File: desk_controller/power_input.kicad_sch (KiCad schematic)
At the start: 14 parts, among them J5 Barrel_Jack_MountingPin, U1 BD95831MUV

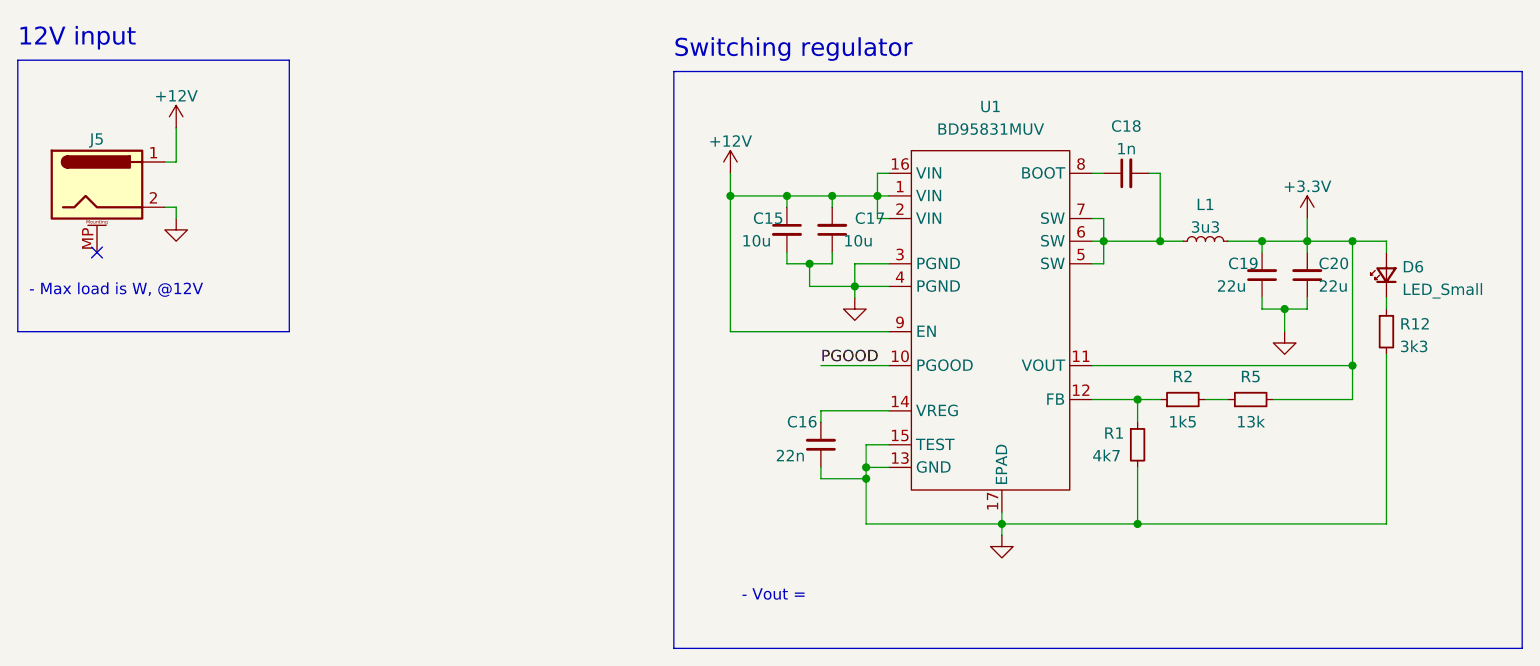
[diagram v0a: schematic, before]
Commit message: Much progress in sch and brd
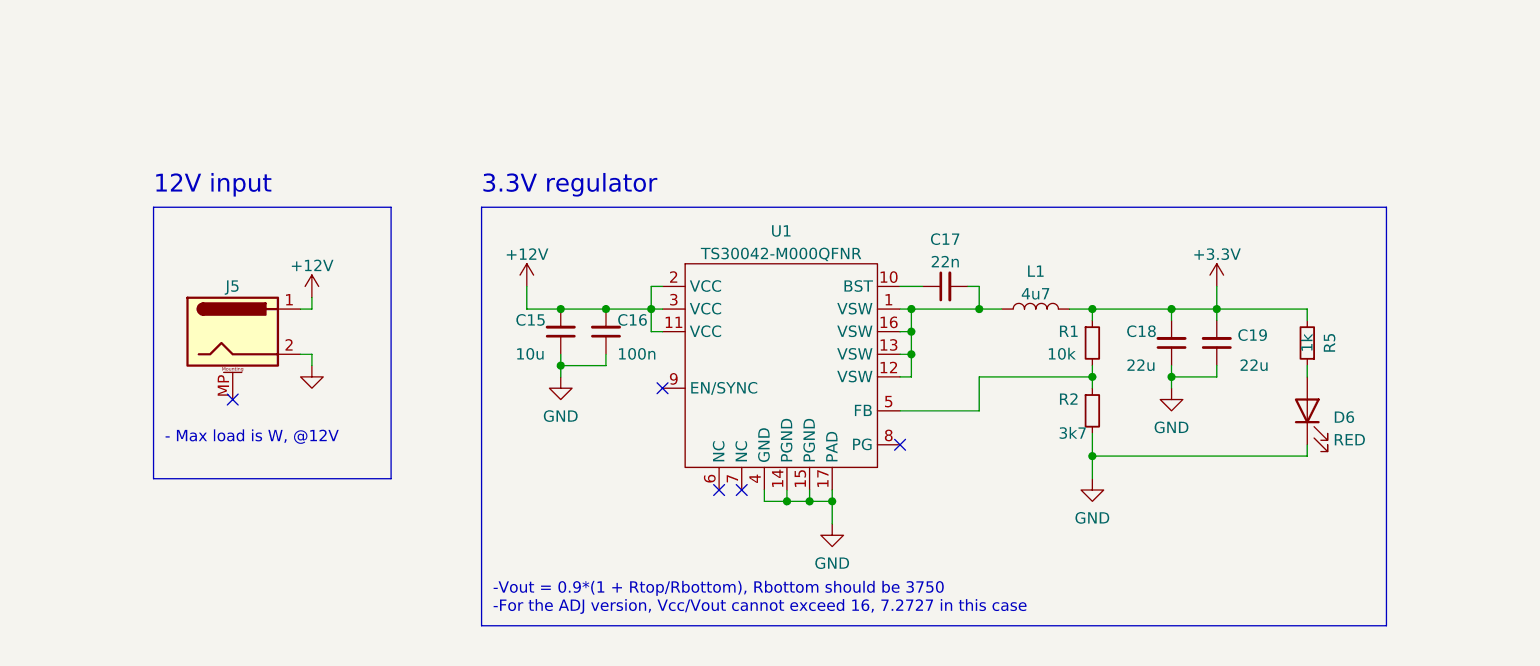
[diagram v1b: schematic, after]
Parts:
- removed C20: 22u, Capacitor_SMD:C_0603_1608Metric, symbol Device:C_Small
- removed D6: LED_Small, symbol Device:LED_Small
- removed L1: 3u3, symbol Device:L_Small
- removed R12: 3k3, Resistor_SMD:R_0603_1608Metric, symbol Device:R_Small
- removed U1: BD95831MUV, Potentiometer_THT:Potentiometer_Bourns_3386F_Vertical, symbol BD95831MUV:BD95831MUV
- added D6: RED, LED_SMD:LED_0603_1608Metric, symbol Device:LED
- added L1: 4u7, BWVS005050404R7M00:BWVS005050404R7M00, symbol Device:L
- added U1: TS30042-M000QFNR, Package_DFN_QFN:QFN-16-1EP_3x3mm_P0.5mm_EP1.75x1.75mm_ThermalVias, symbol TS30042:TS30042
- C15: rating (none) -> 50V
- C16: value 22n -> 100n; rating (none) -> 50V
- C17: value 10u -> 22n
- C18: value 1n -> 22u
- R1: value 4k7 -> 10k
- R2: value 1k5 -> 3k7
- R5: value 13k -> 1k
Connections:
- net +3.3V is gone; now on net +3V3: C19.2, R5.2
- net +12V: now also C15.2, C16.2, U1.11 (VCC), U1.2 (VCC), U1.3 (VCC); no longer C15.1, C17.2
- net GND: now also C15.1, C18.1, R2.2, D6.1 (K), U1.14 (PGND), U1.15 (PGND), U1.17 (PAD), U1.4 (GND); no longer C15.2, C17.1, R1.2
- net at R2.1: now also R1.2, U1.5 (FB); no longer R1.1
- net +3V3: now reaches C18.2
- net +3V3: now also R1.1, L1.2
- net at R5.1: now also D6.2 (A); no longer R2.2
- new net: C17.1, U1.10 (BST)
- new net: C17.2, L1.1, U1.1 (VSW), U1.12 (VSW), U1.13 (VSW), U1.16 (VSW)
- no-connect marks 1 -> 5
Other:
- note added: "-Vout = 0.9*(1 + Rtop/Rbottom), Rbottom should be 3750 -For the ADJ version, Vcc/Vout cannot exceed 16, 7.2727 in this case"
- note added: "3.3V regulator"
- note removed: "- Vout ="
- note removed: "Switching regulator"
- moved on the sheet: J5
